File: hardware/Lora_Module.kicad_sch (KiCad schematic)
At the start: 1 part, among them U7 RFM95W-868S2

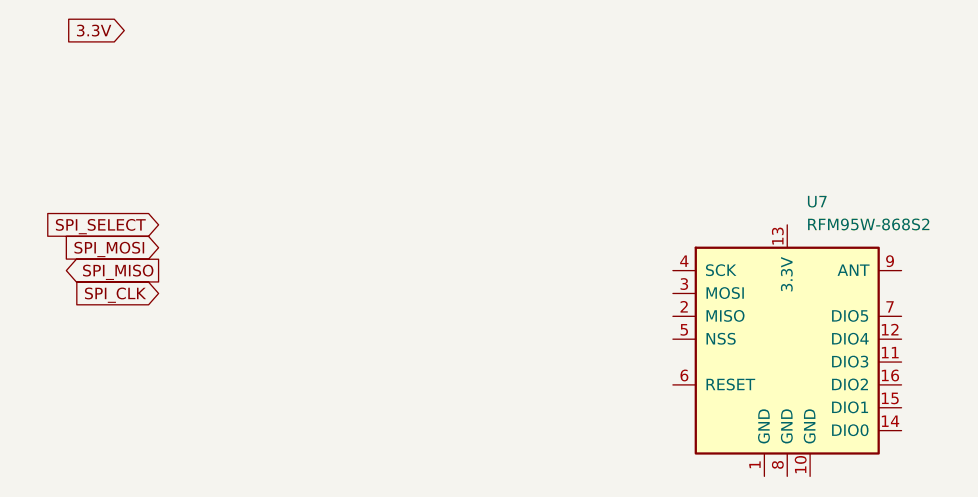
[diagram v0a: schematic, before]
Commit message: GPS schematic + datasheet
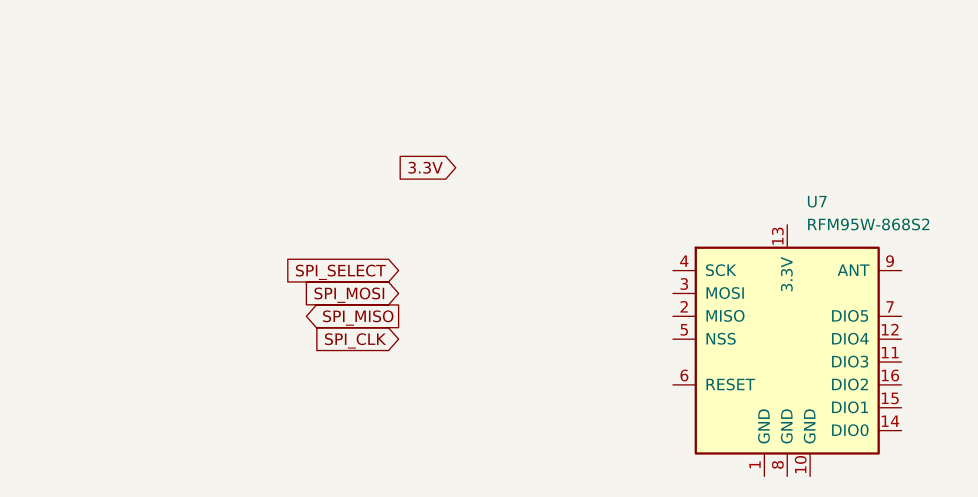
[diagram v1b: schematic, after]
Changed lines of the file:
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@@
 	(global_label "SPI_SELECT"
 		(shape input)
-		(at 39.37 59.69 180)
+		(at 66.04 64.77 180)
 		(fields_autoplaced yes)
 		(effects
@@
 		)
 		(property "Intersheetrefs" "${INTERSHEET_REFS}"
-			(at 25.5597 59.69 0)
+			(at 52.2297 64.77 0)
 			(effects
 				(font
@@
 	(global_label "SPI_MOSI"
 		(shape input)
-		(at 39.37 62.23 180)
+		(at 66.04 67.31 180)
 		(fields_autoplaced yes)
 		(effects
@@
 		)
 		(property "Intersheetrefs" "${INTERSHEET_REFS}"
-			(at 27.7367 62.23 0)
+			(at 54.4067 67.31 0)
 			(effects
 				(font
@@
 	(global_label "3.3V"
 		(shape input)
-		(at 35.56 38.1 180)
+		(at 72.39 53.34 180)
 		(fields_autoplaced yes)
 		(effects
@@
 		)
 		(property "Intersheetrefs" "${INTERSHEET_REFS}"
-			(at 28.4624 38.1 0)
+			(at 65.2924 53.34 0)
 			(effects
 				(font
@@
 	(global_label "SPI_MISO"
 		(shape output)
-		(at 39.37 64.77 180)
+		(at 66.04 69.85 180)
 		(fields_autoplaced yes)
 		(effects
@@
 		)
 		(property "Intersheetrefs" "${INTERSHEET_REFS}"
-			(at 27.7367 64.77 0)
+			(at 54.4067 69.85 0)
 			(effects
 				(font
@@
 	(global_label "SPI_CLK"
 		(shape input)
-		(at 39.37 67.31 180)
+		(at 66.04 72.39 180)
 		(fields_autoplaced yes)
 		(effects
@@
 		)
 		(property "Intersheetrefs" "${INTERSHEET_REFS}"
-			(at 28.7648 67.31 0)
+			(at 55.4348 72.39 0)
 			(effects
 				(font
